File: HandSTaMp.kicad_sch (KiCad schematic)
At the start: 24 parts, among them J1 USB_C_Receptacle_USB2.0_16P, J2 Pins, J3 SWD, SW0 BOOT, SW1 Row 0, Col 0, SW2 Row 0, Col 1, U1 STM32C071GBUx, U2 PRTR5V0U2X, U3 XC6206P332MR-G

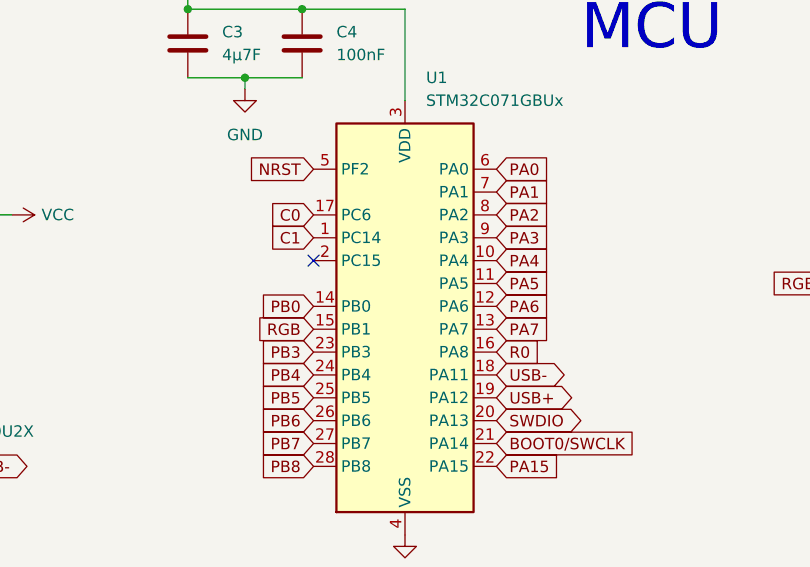
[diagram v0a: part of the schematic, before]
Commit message: Tweak routing, especially R1 and C0
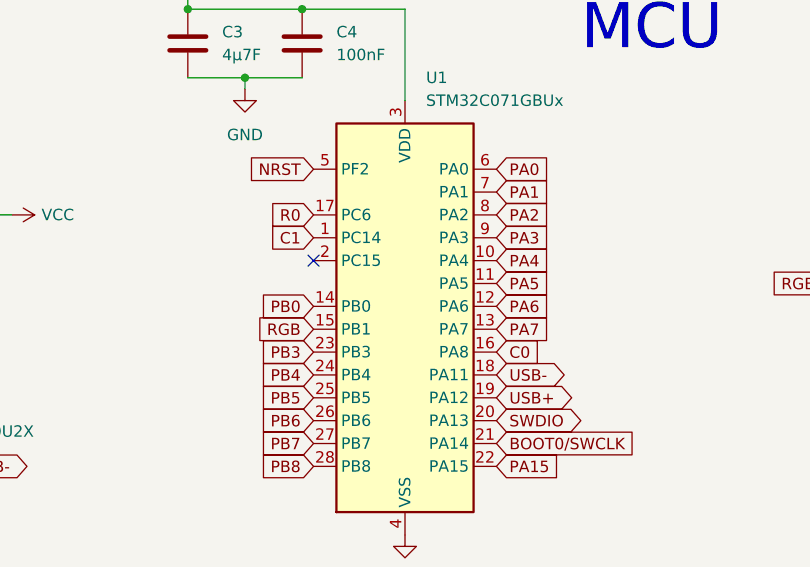
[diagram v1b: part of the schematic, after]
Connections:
- net C0: now also U1.16 (PA8); no longer U1.17 (PC6)
- net R0: now also U1.17 (PC6); no longer U1.16 (PA8)
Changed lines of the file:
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@@
 		)
 	)
-	(global_label "C0"
+	(global_label "R0"
 		(shape input)
 		(at 179.07 40.64 180)
@@
 		)
 		(property "Intersheetrefs" "${INTERSHEET_REFS}"
-			(at 174.3146 40.64 0)
+			(at 174.2029 40.64 0)
 			(hide yes)
 			(show_name no)
@@
 		)
 	)
-	(global_label "R0"
+	(global_label "C0"
 		(shape input)
 		(at 199.39 55.88 0)
@@
 		)
 		(property "Intersheetrefs" "${INTERSHEET_REFS}"
-			(at 204.2571 55.88 0)
-			(hide yes)
-			(show_name no)
+			(at 204.1454 55.88 0)
+			(hide yes)
+			(show_name no)
